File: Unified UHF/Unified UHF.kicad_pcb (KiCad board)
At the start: 2 copper layers, 82.5 x 82.5 mm, 82 parts, among them IC1 QPC1022SR, IC2 GRF5504, IC3 LHA-13LN+, IC4 QPC1022SR, J1 Conn_01x05, J2 Conn_01x02, J3 Conn_01x02, J4 Conn_01x01, J5 PCB.SMAFST.2H.A.HT, U1 AT86RF215-ZU, U2 NCS-62+, X1 TYETACSANF-26.000000

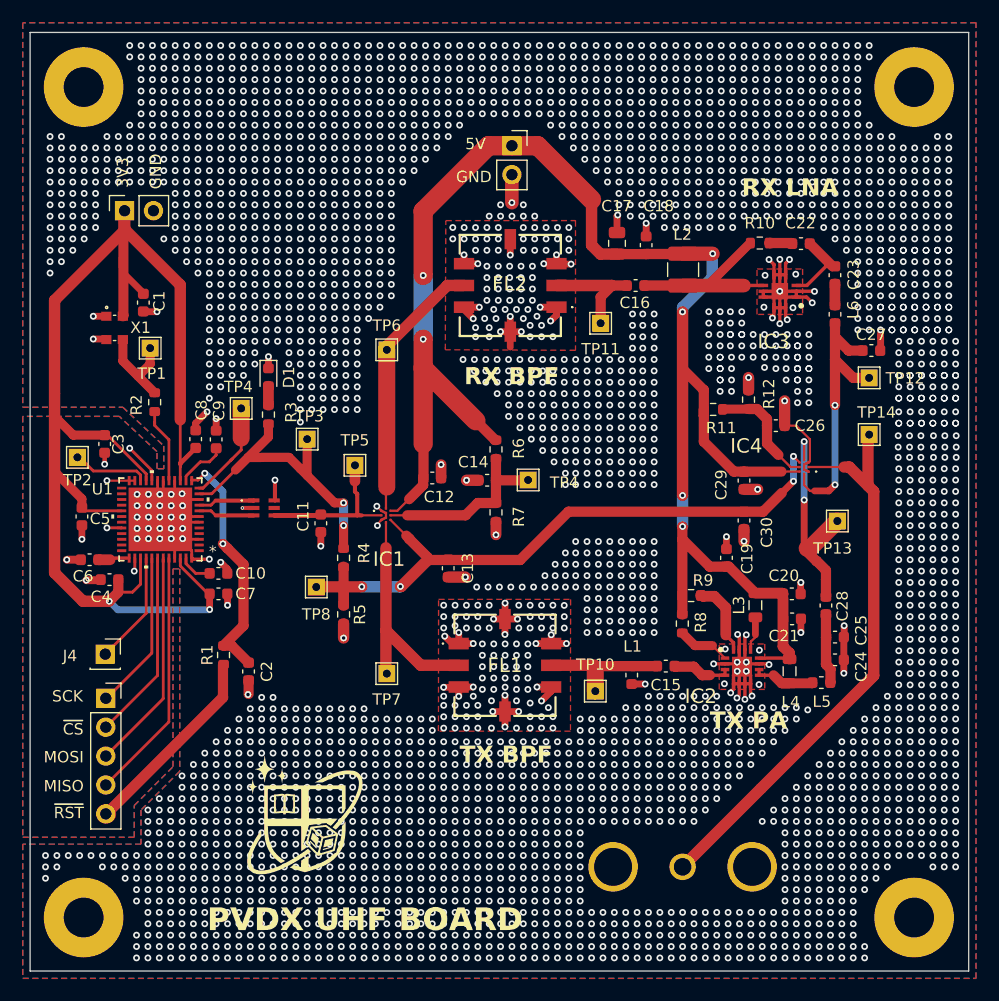
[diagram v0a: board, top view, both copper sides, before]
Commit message: pad sizing, vias, checking things, etc
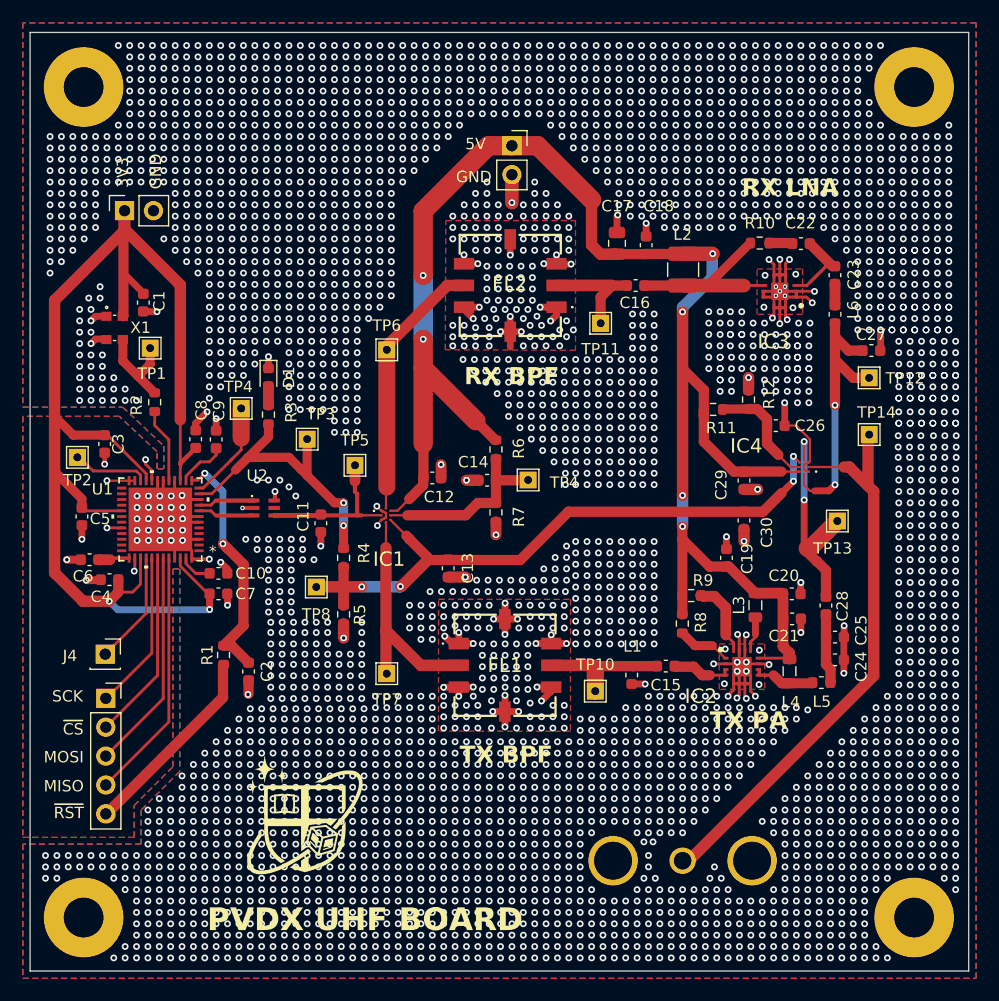
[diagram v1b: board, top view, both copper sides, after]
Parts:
- moved J5 0.54 mm to (88.2, 90.8)
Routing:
- net GND: track 173.4 -> 172.3 mm, vias 3550 -> 3878
- net Net-(IC2-VCC1): track 2.98 -> 3.66 mm
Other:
- board text added: "U2"

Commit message: before updating from schematic - as for as I know this is good
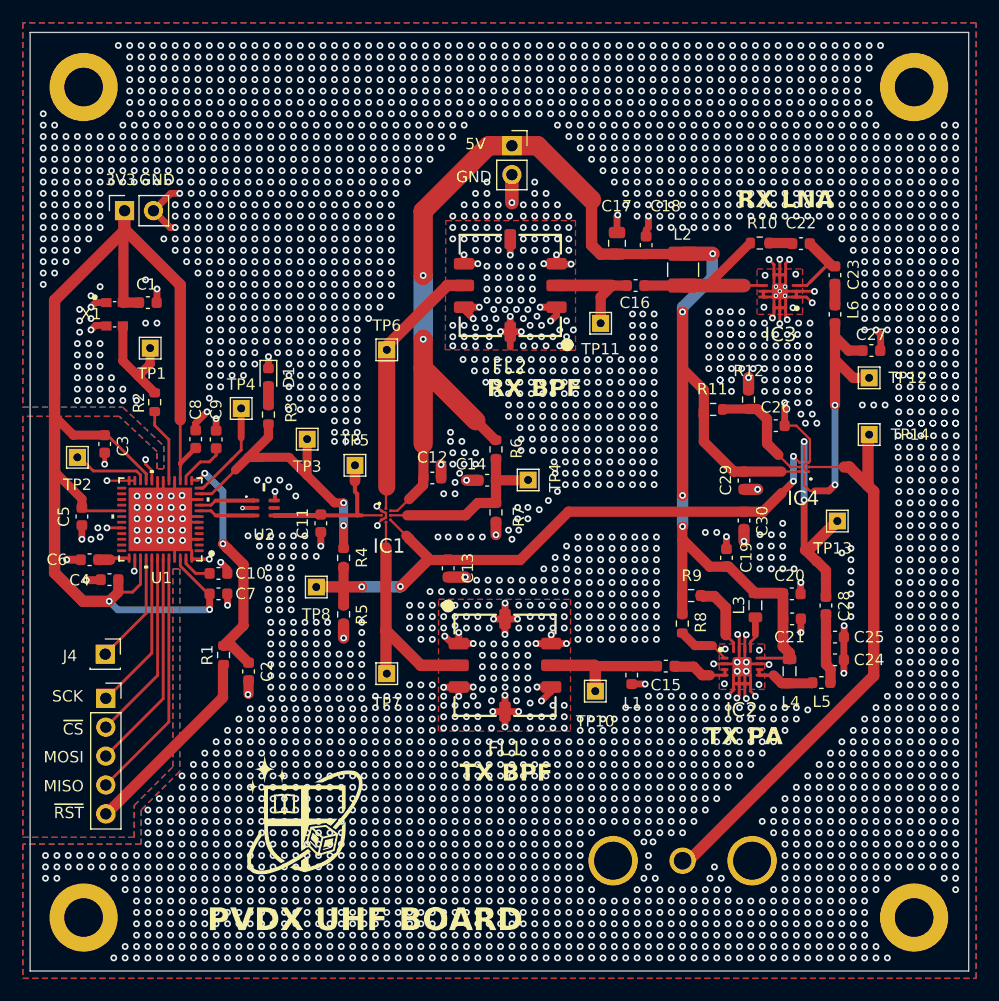
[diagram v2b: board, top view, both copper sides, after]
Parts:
- C19, C20, C22: value 0.1u -> 100n
- U1: footprint AT86RF215:QFN48_PQ_MCH -> RF Frontend Footprints:AT86Footprint
- moved X1 1.20 mm to (43.3, 42.8)
- moved C1 0.40 mm to (41.2, 41.8), turned to 180 degrees
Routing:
- net GND: track 172.3 -> 178.6 mm, vias 3878 -> 3969
- net +3V3: track 123.0 -> 120.6 mm
- net Net-(X1-OUT): track 8.39 -> 9.94 mm

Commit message: done prob
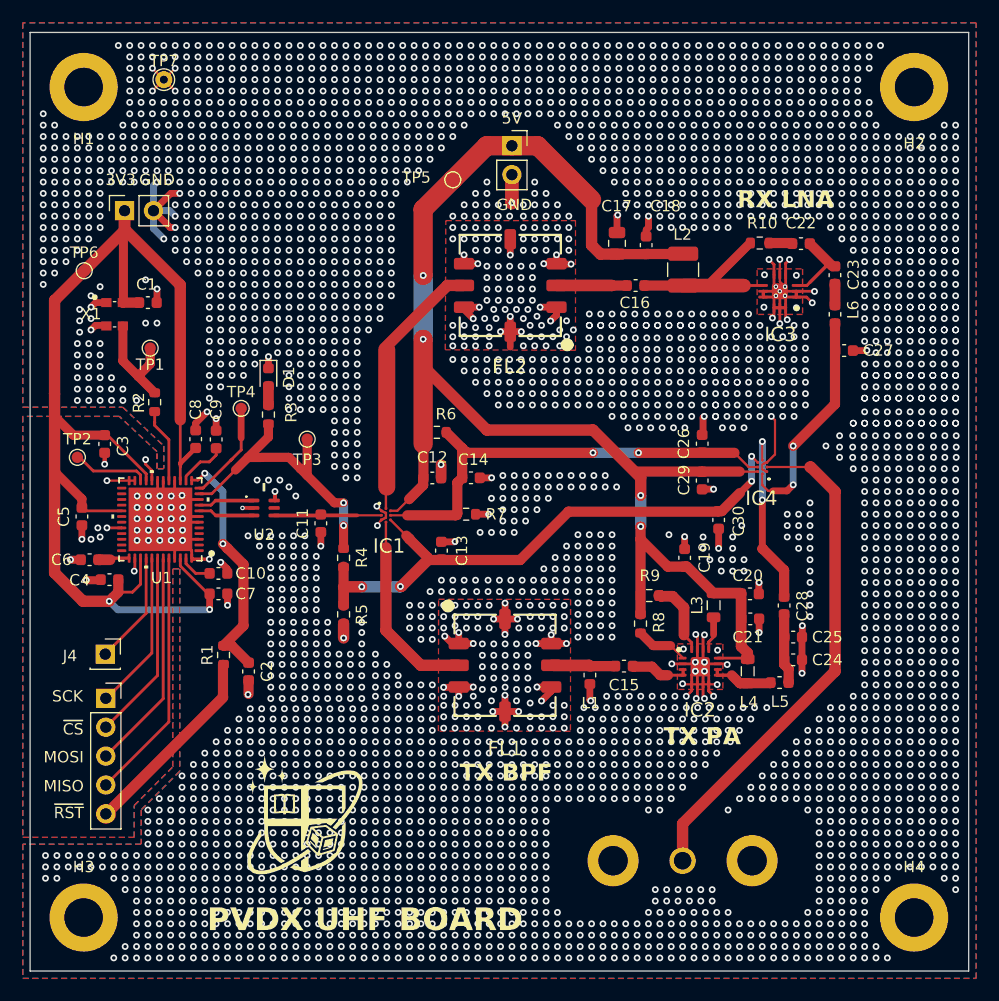
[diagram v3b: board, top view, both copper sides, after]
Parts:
- removed R11: 10k, Resistor_SMD:R_0603_1608Metric
- removed R12: 5.6k, Resistor_SMD:R_0603_1608Metric
- removed TP10, TP11, TP12, TP13, TP14, TP8, TP9: TestPoint, TestPoint:TestPoint_THTPad_1.5x1.5mm_Drill0.7mm
- H1, H2, H3, H4: footprint MountingHole:MountingHole_3.5mm_Pad -> RF Frontend Footprints:MountingHole_3.4mm_Pad(edited from 3.5mm hole)
- TP1, TP2, TP3, TP4, TP5, TP6: footprint TestPoint:TestPoint_THTPad_1.5x1.5mm_Drill0.7mm -> TestPoint:TestPoint_Pad_D1.0mm
- TP7: footprint TestPoint:TestPoint_THTPad_1.5x1.5mm_Drill0.7mm -> TestPoint:TestPoint_THTPad_D1.5mm_Drill0.7mm
- moved TP7 55.8 mm to (42.6, 22.2)
- moved TP6 27.5 mm to (35.6, 39.0)
- moved TP5 26.5 mm to (68.0, 31.0), turned to 0 degrees
- moved C26 6.66 mm to (89.9, 54.2), turned to 90 degrees
- moved R6 5.41 mm to (66.6, 53.2), turned to 0 degrees
- moved C15 3.68 mm to (83.1, 73.7)
- moved C19 3.68 mm to (88.4, 64.2)
- moved C20 3.68 mm to (94.1, 67.4)
- moved C21 3.68 mm to (94.2, 69.6)
- moved C24 3.68 mm to (97.9, 73.2)
- moved C25 3.68 mm to (97.9, 71.2)
- moved C28 3.68 mm to (97.1, 68.4)
- moved IC2 3.68 mm to (89.8, 73.8)
- moved IC4 3.68 mm to (95.2, 56.2)
- moved L1 3.68 mm to (80.1, 74.5)
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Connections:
- C26 pad 1: Net-(IC4-EN) -> Net-(IC1-EN)
- IC4 pad 6: Net-(IC4-EN) -> Net-(IC1-EN)
- TP5 pad 1: Net-(IC1-ANT) -> +5V
- TP6 pad 1: Net-(FL2-RF_OUT) -> +3V3
- TP7 pad 1: Net-(FL1-RF_IN) -> GND
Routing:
- net Net-(IC1-EN): track 16.6 -> 40.7 mm, vias 0 -> 2
- net +5V: track 141.3 -> 125.7 mm, vias 6 -> 4
- net GND: track 178.6 -> 189.5 mm, vias 3969 -> 3979
- net Net-(IC4-EN): track 10.8 -> 0.00 mm
- net Net-(IC1-ANT): track 18.0 -> 9.55 mm
- net Net-(IC4-ANT): track 51.1 -> 44.9 mm
- net Net-(IC1-CTRL): track 57.1 -> 51.0 mm
- net Net-(IC4-RF2): track 24.9 -> 19.9 mm
- net Net-(IC4-RF1): track 19.9 -> 16.1 mm
- net Net-(FL1-RF_IN): track 20.9 -> 17.2 mm
- net Net-(FL2-RF_IN): track 9.89 -> 6.16 mm
- net Net-(FL1-RF_OUT): track 11.4 -> 9.10 mm
- net +3V3: track 120.6 -> 119.7 mm
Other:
- board text removed: "RX BPF"
- board text removed: "TP4"

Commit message: finally done
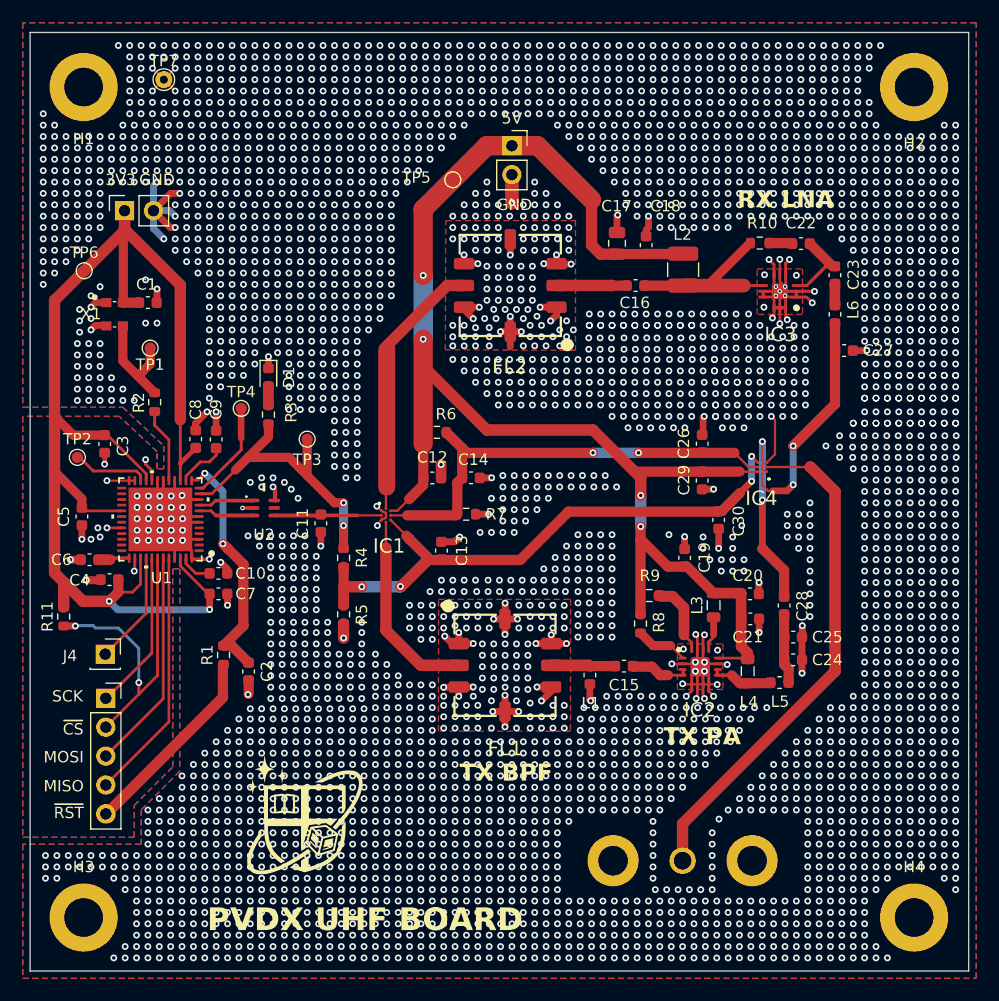
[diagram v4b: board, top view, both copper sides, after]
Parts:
- added R11: 10k, Resistor_SMD:R_0603_1608Metric, F.Cu at (33.8, 69.4)
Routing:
- net Net-(J1-Pin_2): track 16.7 -> 28.2 mm, vias 0 -> 2
- net +3V3: track 119.7 -> 121.9 mm
- net GND: track 189.5 -> 191.1 mm, vias 3979 -> 4052
- net Net-(IC4-RF2): track 19.9 -> 21.2 mm

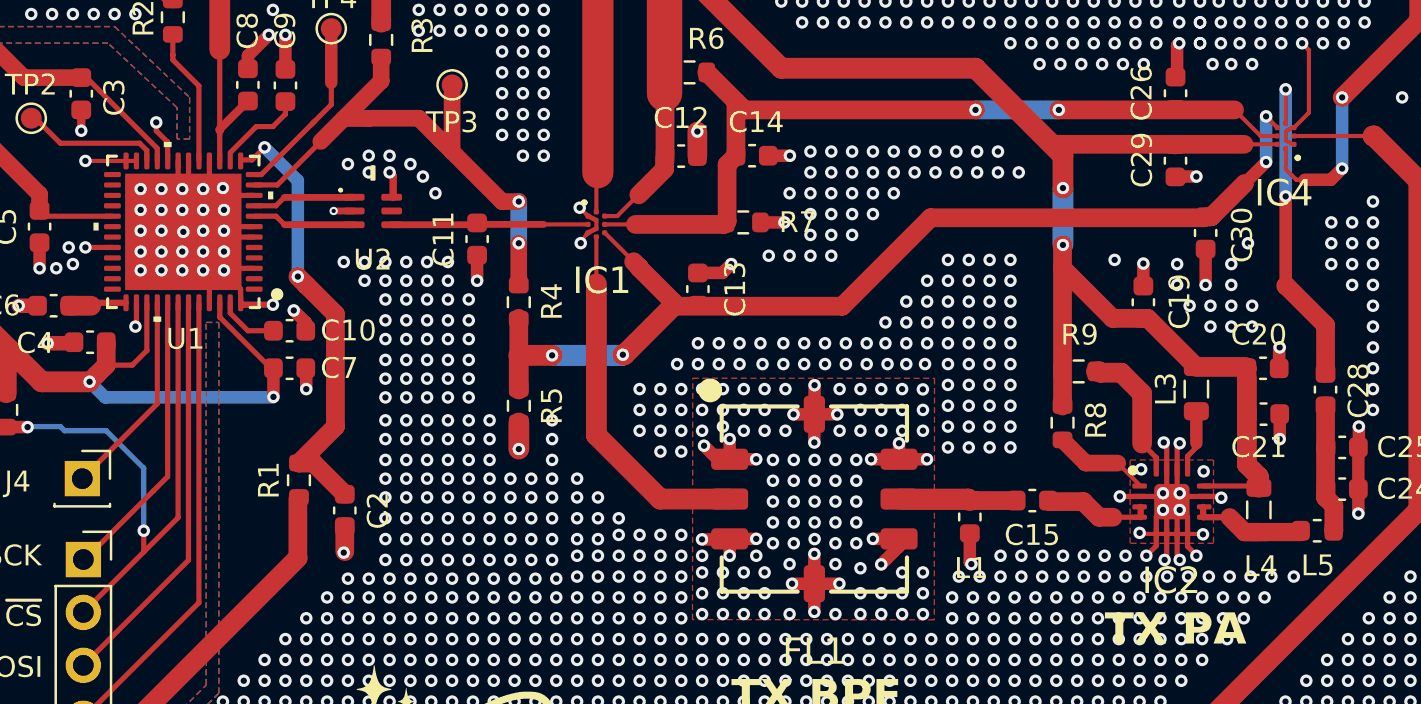
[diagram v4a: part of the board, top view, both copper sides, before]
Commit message: small pcbway tweaks
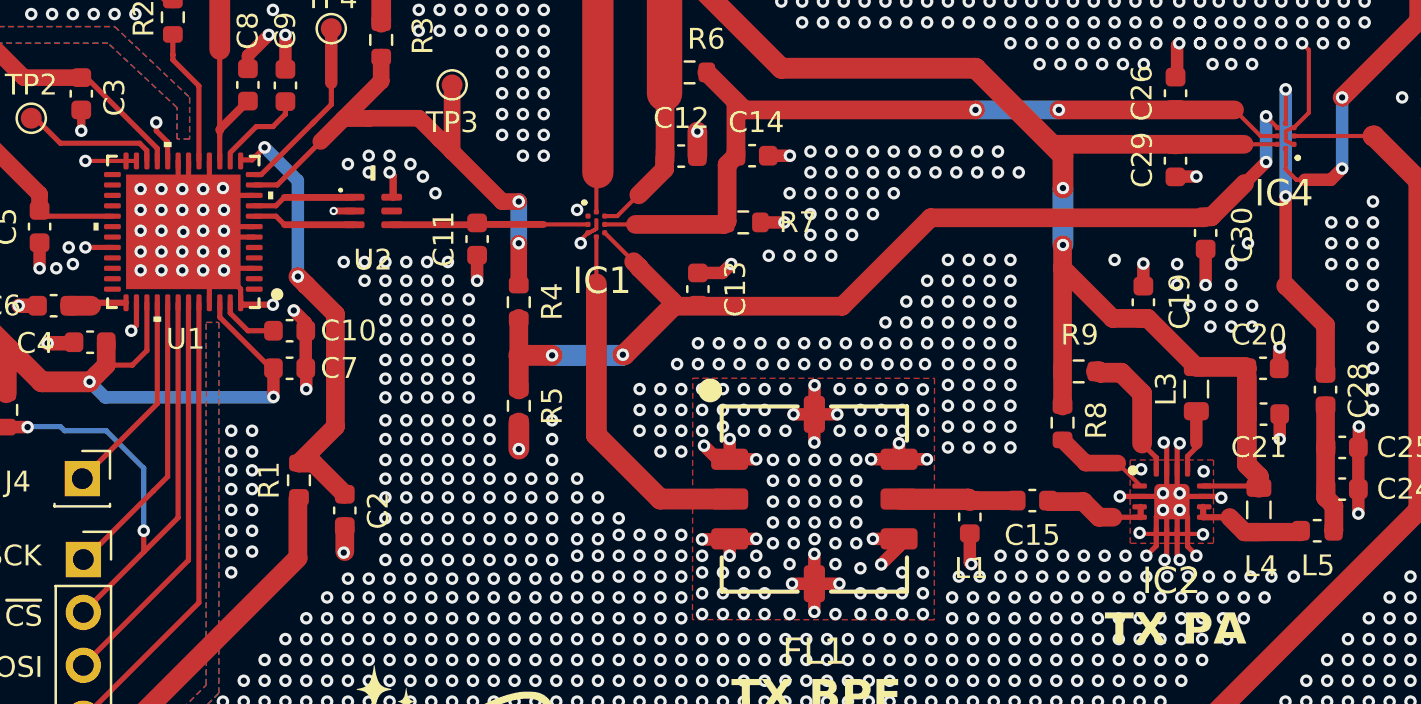
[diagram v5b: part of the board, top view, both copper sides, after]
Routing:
- net GND: track 191.1 -> 193.9 mm, vias 4052 -> 4067
